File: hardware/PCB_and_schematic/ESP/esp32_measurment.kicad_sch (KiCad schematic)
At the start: 104 parts, among them J1 DB9_Socket, J13 H2_SENSOR, J14 7SEG_DISP, J15 CO_SENSOR, J17 LCD_DISP, J20 DHT22, J3 BATTERY_SHUNT, J4 DC_LINE_OUTPUT, J6 RS485, J8 OR_OR_Smoke_sensor, K1 Relay_SPST-NO, Q1 BSS138, Q2 BSS138, Q3 BC817, Q4 BC817, Q5 BC817, Q6 BC817, Q7 BC817, Q8 NPN, Q9 BC817, SW1 SW_Push, U1 ESP32_DevKit_V1_DOIT, U10 UP7760, U19 PCF8574, U2 INA226, U3 MAX232, U7 AMS1117-5.0, U8 ST485, U9 INA226

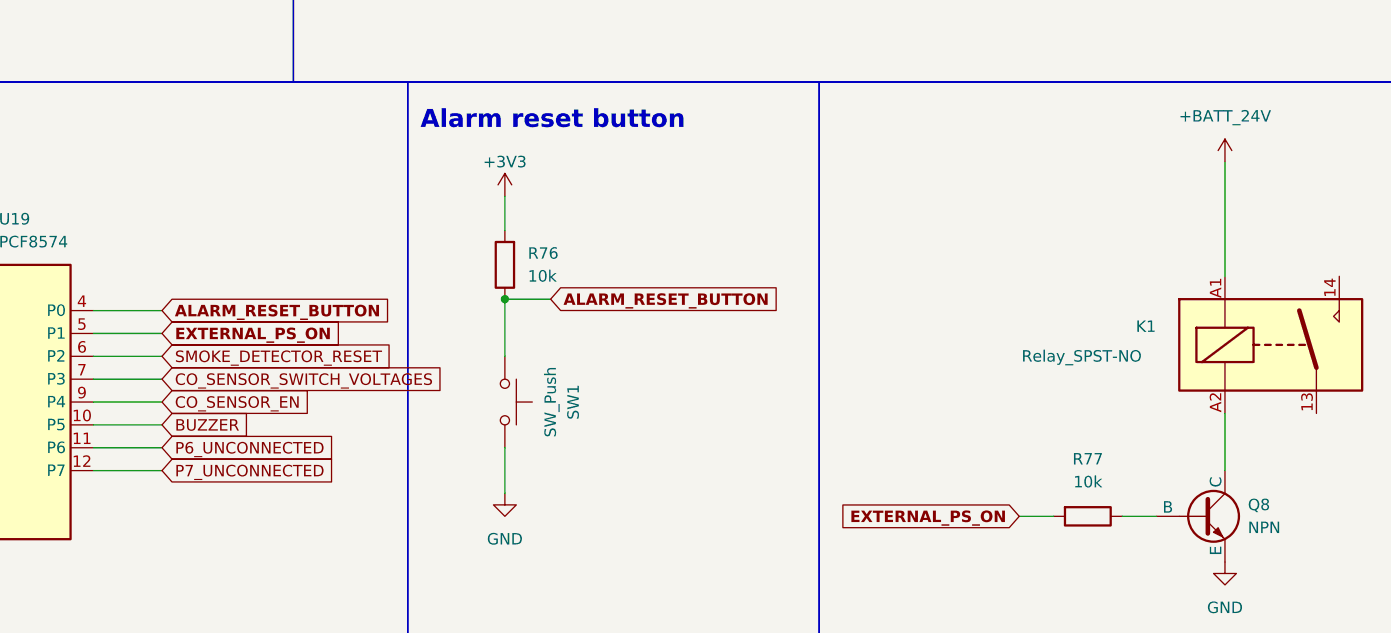
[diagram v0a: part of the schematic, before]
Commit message: corase routing for esp doce
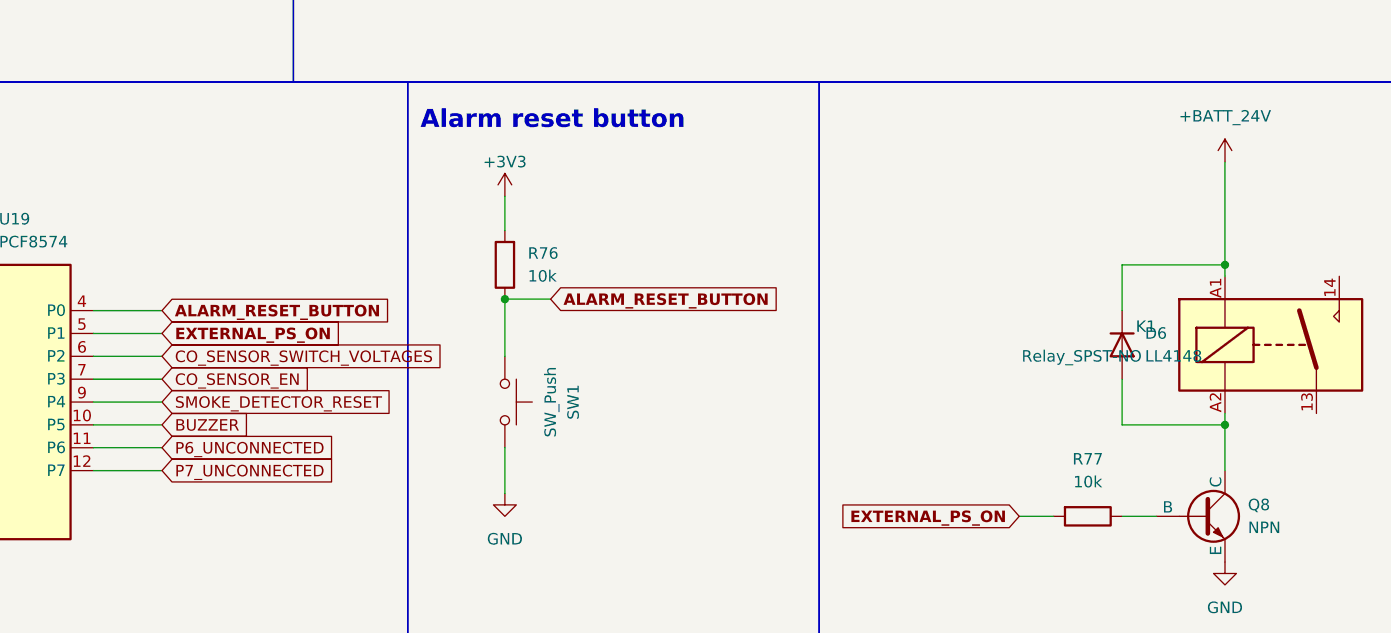
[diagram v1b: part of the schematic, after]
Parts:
- added D6: LL4148, Diode_SMD:D_MiniMELF, symbol Diode:LL4148
- Q8: footprint Package_TO_SOT_THT:TO-92_Inline_Wide -> My-Footprints:TO-92_Inline_Wide
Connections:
- net +BATT_24V: now also D6.1 (K)
- net CO_SENSOR_EN: now also U19.7 (P3); no longer U19.9 (P4)
- net CO_SENSOR_SWITCH_VOLTAGES: now also U19.6 (P2); no longer U19.7 (P3)
- net SMOKE_DETECTOR_RESET: now also U19.9 (P4); no longer U19.6 (P2)
- net at K1.A2, Q8.1 (C): now also D6.2 (A)
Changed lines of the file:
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@@
 	)
 	(junction
+		(at 219.71 248.92)
+		(diameter 0)
+		(color 0 0 0 0)
+	)
+	(junction
 		(at 288.29 250.19)
 		(diameter 0)
@@
 	)
 	(junction
+		(at 219.71 266.7)
+		(diameter 0)
+		(color 0 0 0 0)
+	)
+	(junction
 		(at 199.39 194.31)
 		(diameter 0)
@@
 	(wire
 		(pts
+			(xy 208.28 254) (xy 208.28 248.92)
+		)
+		(stroke
+			(width 0)
+			(type default)
+		)
+	)
+	(wire
+		(pts
 			(xy 397.51 90.17) (xy 401.32 90.17)
 		)
@@
 	(wire
 		(pts
-			(xy 219.71 237.49) (xy 219.71 250.19)
+			(xy 219.71 237.49) (xy 219.71 248.92)
 		)
 		(stroke
@@
 	(wire
 		(pts
-			(xy 219.71 265.43) (xy 219.71 271.78)
+			(xy 219.71 265.43) (xy 219.71 266.7)
 		)
 		(stroke
@@
 	(wire
 		(pts
+			(xy 219.71 266.7) (xy 219.71 271.78)
+		)
+		(stroke
+			(width 0)
+			(type default)
+		)
+	)
+	(wire
+		(pts
 			(xy 232.41 101.6) (xy 232.41 91.44)
 		)
@@
 	(wire
 		(pts
+			(xy 208.28 266.7) (xy 208.28 261.62)
+		)
+		(stroke
+			(width 0)
+			(type default)
+		)
+	)
+	(wire
+		(pts
 			(xy 422.91 161.29) (xy 429.26 161.29)
 		)
@@
 	(wire
 		(pts
+			(xy 208.28 248.92) (xy 219.71 248.92)
+		)
+		(stroke
+			(width 0)
+			(type default)
+		)
+	)
+	(wire
+		(pts
 			(xy 397.51 207.01) (xy 402.59 207.01)
 		)
@@
 	(wire
 		(pts
+			(xy 219.71 266.7) (xy 208.28 266.7)
+		)
+		(stroke
+			(width 0)
+			(type default)
+		)
+	)
+	(wire
+		(pts
 			(xy 316.23 147.32) (xy 304.8 147.32)
 		)
@@
 	(wire
 		(pts
+			(xy 219.71 248.92) (xy 219.71 250.19)
+		)
+		(stroke
+			(width 0)
+			(type default)
+		)
+	)
+	(wire
+		(pts
 			(xy 527.05 160.02) (xy 527.05 163.83)
 		)
@@
 	(global_label "SMOKE_DETECTOR_RESET"
 		(shape input)
-		(at 101.6 259.08 0)
+		(at 101.6 264.16 0)
 		(fields_autoplaced yes)
 		(effects
@@
 		)
 		(property "Intersheetrefs" "${INTERSHEET_REFS}"
-			(at 128.0496 259.08 0)
+			(at 128.0496 264.16 0)
 			(effects
 				(font
@@
 	(global_label "CO_SENSOR_SWITCH_VOLTAGES"
 		(shape input)
-		(at 101.6 261.62 0)
+		(at 101.6 259.08 0)
 		(fields_autoplaced yes)
 		(effects
@@
 		)
 		(property "Intersheetrefs" "${INTERSHEET_REFS}"
-			(at 133.5532 261.62 0)
+			(at 133.5532 259.08 0)
 			(effects
 				(font
@@
 	(global_label "CO_SENSOR_EN"
 		(shape input)
-		(at 101.6 264.16 0)
+		(at 101.6 261.62 0)
 		(fields_autoplaced yes)
 		(effects
@@
 		)
 		(property "Intersheetrefs" "${INTERSHEET_REFS}"
-			(at 119.0994 264.16 0)
+			(at 119.0994 261.62 0)
 			(effects
 				(font
@@
 			)
 		)
-		(property "Footprint" "Package_TO_SOT_THT:TO-92_Inline_Wide"
+		(property "Footprint" "My-Footprints:TO-92_Inline_Wide"
 			(at 280.67 276.86 0)
 			(effects
@@
 					(unit 1)
 				)
+			)
+		)
+	)
+	(symbol
+		(lib_id "Diode:LL4148")
+		(at 208.28 257.81 270)
+		(unit 1)
+		(exclude_from_sim no)
+		(in_bom yes)
+		(on_board yes)
+		(dnp no)
+		(fields_autoplaced yes)
+		(property "Reference" "D6"
+			(at 210.82 256.5399 90)
+			(effects
+				(font
+					(size 1.27 1.27)
+				)
+				(justify left)
+			)
+		)
+		(property "Value" "LL4148"
+			(at 210.82 259.0799 90)
+			(effects
+				(font
+					(size 1.27 1.27)
+				)
+				(justify left)
+			)
+		)
+		(property "Footprint" "Diode_SMD:D_MiniMELF"
+			(at 203.835 257.81 0)
+			(effects
+				(font
+					(size 1.27 1.27)
+				)
+				(hide yes)
+			)
+		)
+		(property "Datasheet" "http://www.vishay.com/docs/85557/ll4148.pdf"
+			(at 208.28 257.81 0)
+			(effects
+				(font
+					(size 1.27 1.27)
+				)
+				(hide yes)
+			)
+		)
+		(property "Description" "100V 0.15A standard switching diode, MiniMELF"
+			(at 208.28 257.81 0)
+			(effects
+				(font
+					(size 1.27 1.27)
+				)
+				(hide yes)
+			)
+		)
+		(property "Sim.Device" "D"
+			(at 208.28 257.81 0)
+			(effects
+				(font
+					(size 1.27 1.27)
+				)
+				(hide yes)
+			)
+		)
+		(property "Sim.Pins" "1=K 2=A"
+			(at 208.28 257.81 0)
+			(effects
+				(font
+					(size 1.27 1.27)
+				)
+				(hide yes)
+			)
+		)
+		(pin "1"
+		)
+		(pin "2"
+		)
+		(instances
+			(project "ESP32_master"
+				(path "/555ba40f-9abb-4b99-82c6-07e888fda9fd/a8064d67-baba-4afe-84af-1260f43bc5ee"
+					(reference "D6")
+					(unit 1)
+				)
